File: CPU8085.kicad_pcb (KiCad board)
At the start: 2 copper layers, 100 x 100 mm, 52 parts, among them J1 USB_B, J2 SPEAKER, Q1 BC817, Q2 IRLML6402, SW1 RESET, U1 GLUE_LOGIC, U2 27C256, U3 IS61C256AH, U4 8250, U5 FT232RL, U6 82C54, U7 8085, U8 74LS573, Y1 4MHz

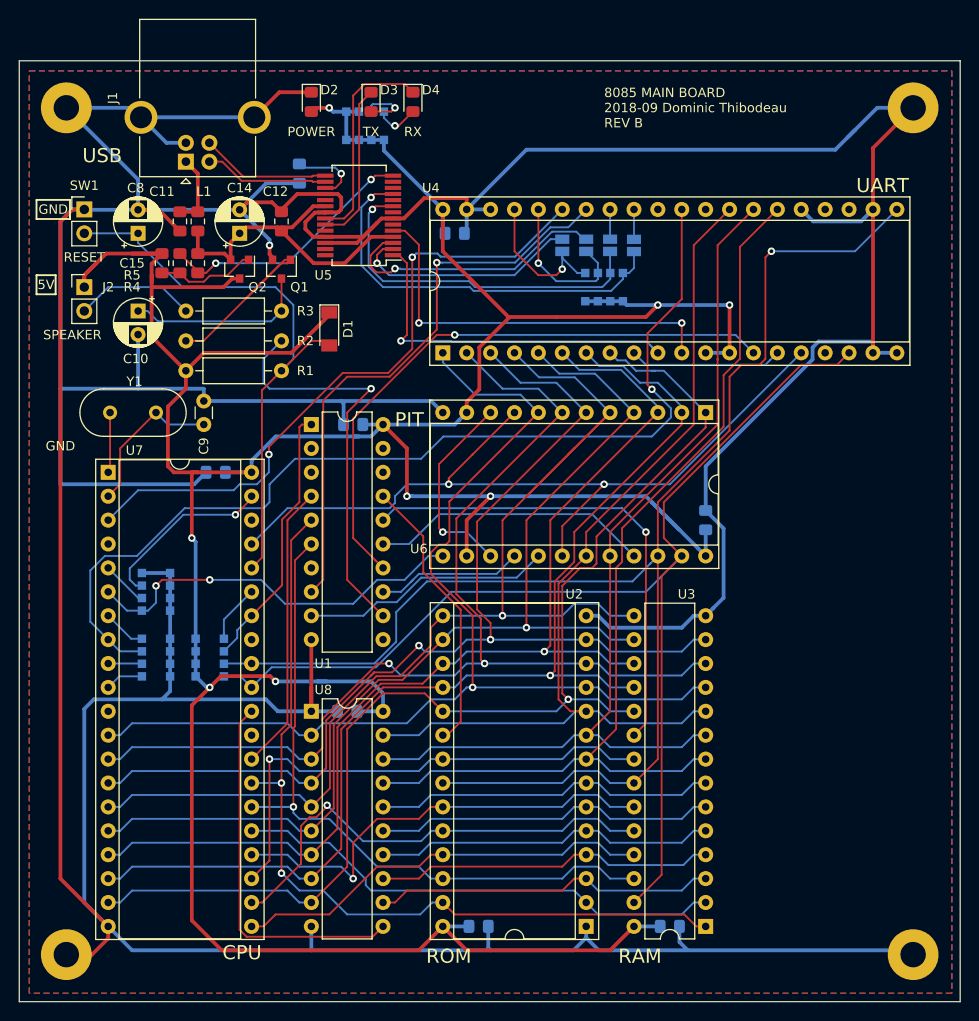
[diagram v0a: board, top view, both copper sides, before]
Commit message: RevC
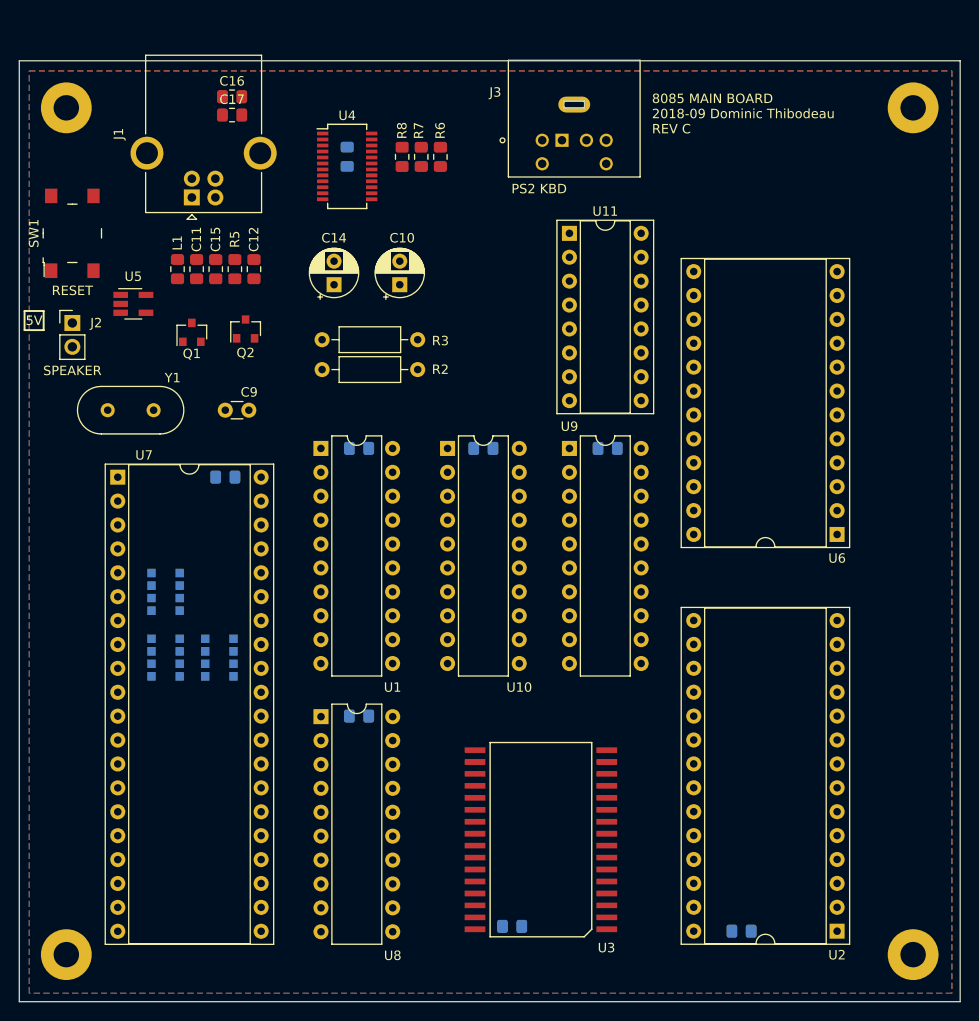
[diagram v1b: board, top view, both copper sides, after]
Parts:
- removed C8: 1uF, Capacitor_THT:CP_Radial_D5.0mm_P2.50mm
- removed D1: 1N4004, Diode_SMD:D_MiniMELF
- removed D2: POWER, LED_SMD:LED_0805_2012Metric_Pad1.15x1.40mm_HandSolder
- removed D3: TX, LED_SMD:LED_0805_2012Metric_Pad1.15x1.40mm_HandSolder
- removed D4: RX, LED_SMD:LED_0805_2012Metric_Pad1.15x1.40mm_HandSolder
- removed JP1: ~DTR, Jumper:SolderJumper-2_P1.3mm_Open_Pad1.0x1.5mm
- removed JP2: ~RTS, Jumper:SolderJumper-2_P1.3mm_Open_Pad1.0x1.5mm
- removed JP3: ~DSR, Jumper:SolderJumper-2_P1.3mm_Open_Pad1.0x1.5mm
- removed JP4: ~CTS, Jumper:SolderJumper-2_P1.3mm_Open_Pad1.0x1.5mm
- removed R1: 75K, Resistor_THT:R_Axial_DIN0207_L6.3mm_D2.5mm_P10.16mm_Horizontal
- removed R4: 10K, Resistor_SMD:R_0805_2012Metric_Pad1.15x1.40mm_HandSolder
- removed RN3: 10K, Resistor_SMD:R_Array_Convex_4x1206
- removed RN5: 330, Resistor_SMD:R_Array_Convex_4x1206
- added C16: 47pF, Capacitor_SMD:C_0805_2012Metric_Pad1.15x1.40mm_HandSolder, F.Cu at (57.6, 38.8)
- added C17: 47pF, Capacitor_SMD:C_0805_2012Metric_Pad1.15x1.40mm_HandSolder, F.Cu at (57.6, 40.8)
- added J3: PS2 KBD, 8085:CUI_MD-60S, F.Cu at (94.0, 41.1)
- added R6: 27R, Resistor_SMD:R_0805_2012Metric_Pad1.15x1.40mm_HandSolder, F.Cu at (79.8, 45.2)
- added R7: 27R, Resistor_SMD:R_0805_2012Metric_Pad1.15x1.40mm_HandSolder, F.Cu at (77.7, 45.2)
- added R8: 10K, Resistor_SMD:R_0805_2012Metric_Pad1.15x1.40mm_HandSolder, F.Cu at (75.7, 45.2)
- added U10: 74LS573, Package_DIP:DIP-20_W7.62mm, F.Cu at (80.5, 76.2)
- added U11: SN76489, Package_DIP:DIP-16_W7.62mm_Socket, F.Cu at (93.5, 53.3)
- added U9: DTBANK1, Package_DIP:DIP-20_W7.62mm, F.Cu at (93.5, 76.2)
- C12, C13: value 0.1uF -> 100nF
- C14: value 1uF -> 4.7uF
- SW1: footprint Connector_PinHeader_2.54mm:PinHeader_1x02_P2.54mm_Vertical -> 8085:Switch_Tactile_SMD_6x6mm_PTS645
- U1: value GLUE_LOGIC -> DTGLUE4
- U3: value IS61C256AH -> IS62C1024AL; footprint Package_DIP:DIP-28_W7.62mm -> 8085:SOIC-32W_14x21mm_P1.27mm
- U4: value 8250 -> FT240XS; footprint Package_DIP:DIP-40_W15.24mm_Socket -> Package_SO:SSOP-24_3.9x8.7mm_P0.635mm
- U5: value FT232RL -> MCP1319T-46LE; footprint Package_SO:SSOP-28_5.3x10.2mm_P0.65mm -> Package_TO_SOT_SMD:SOT-23-5_HandSoldering
- moved C4 67.8 mm to (111.8, 127.5), turned to 0 degrees
- moved C2 52.6 mm to (97.5, 76.2), turned to 180 degrees
- moved C6 37.6 mm to (71.1, 76.2), turned to 180 degrees
- moved C7 30.1 mm to (71.1, 104.6)
- moved C5 28.1 mm to (56.9, 79.2)
- moved C10 28.0 mm to (75.4, 58.8), turned to 90 degrees
- moved U2 26.7 mm to (121.9, 127.5)
- moved U5 25.8 mm to (47.1, 60.8), turned to 0 degrees
- moved R3 24.8 mm to (77.3, 64.6), turned to 180 degrees
- moved C1 23.1 mm to (84.3, 76.2), turned to 180 degrees
- moved U4 22.3 mm to (69.8, 46.2), turned to 0 degrees
- moved U3 19.8 mm to (90.4, 117.9)
- moved U6 19.1 mm to (121.9, 85.3), turned to 180 degrees
- moved C3 16.8 mm to (87.4, 127.0)
- moved R2 14.8 mm to (67.2, 67.8)
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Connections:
- net /UART/VIN renamed /UART (FT240XS)/VIN
- J1 pad 2: /UART/D- -> /UART (FT240XS)/D-
- J1 pad 3: /UART/D+ -> /UART (FT240XS)/D+
- R2 pad 2: /SPEAKER/SPKR_IN -> Net-(R2-Pad2)
- R5 pad 2: /UART/~PWREN -> /UART (FT240XS)/~PWREN
- RN1 pad 5: /PIT/TI_CLK -> /CPU/TRAP
- RN2 pad 7: /UART/INTR -> /CPU/RST6_5
- SW1 pad 2: Net-(C8-Pad1) -> Net-(SW1-Pad2)
- U1 pad 12: /SPEAKER/SPKR_IN -> (no net)
- U1 pad 13: /PIT/SPKR_EN -> (no net)
- U1 pad 14: /UART/~UART -> (no net)
- U1 pad 15: /PIT/~PIT -> /Sound (SN76489)/~SOUND
- U1 pad 16: /Memory/~RAMCE -> /UART (FT240XS)/~UART_RD
- U1 pad 17: /Memory/~ROMCE -> /UART (FT240XS)/UART_WR
- U1 pad 18: (no net) -> /PIT/~PIT
- U1 pad 19: (no net) -> /Memory/BANKREG
- U1 pad 2: (no net) -> /A15
- U1 pad 3: (no net) -> /A14
- U1 pad 4: /A15 -> /A13
- U1 pad 5: /A14 -> /CPU/~WR
- U1 pad 6: /A13 -> /CPU/~RD
- U1 pad 8: /UART/~UART_OUT1 -> (no net)
- U1 pad 9: /PIT/SPKR_OUT -> (no net)
- U3 pad 1: /A14 -> (no net)
- U3 pad 10: /CPU/A0 -> /CPU/A2
- U3 pad 11: /CPU/D0 -> /CPU/A1
- U3 pad 12: /CPU/D1 -> /CPU/A0
- U3 pad 13: /CPU/D2 -> /CPU/D0
- U3 pad 14: GND -> /CPU/D1
- U3 pad 15: /CPU/D3 -> /CPU/D2
- U3 pad 16: /CPU/D4 -> GND
- U3 pad 17: /CPU/D5 -> /CPU/D3
- U3 pad 18: /CPU/D6 -> /CPU/D4
- U3 pad 19: /CPU/D7 -> /CPU/D5
- U3 pad 2: /CPU/A12 -> /Memory/RAMA16
- U3 pad 20: /Memory/~RAMCE -> /CPU/D6
- U3 pad 21: /CPU/A10 -> /CPU/D7
- U3 pad 22: /CPU/~RD -> /Memory/~RAMCE
- U3 pad 23: /CPU/A11 -> /CPU/A10
- U3 pad 24: /CPU/A9 -> /CPU/~RD
- U3 pad 25: /CPU/A8 -> /CPU/A11
- U3 pad 26: /A13 -> /CPU/A9
- U3 pad 27: /CPU/~WR -> /CPU/A8
- U3 pad 28: VCC -> /Memory/RAMA13
- U3 pad 3: /CPU/A7 -> /Memory/RAMA14
- U3 pad 4: /CPU/A6 -> /CPU/A12
- U3 pad 5: /CPU/A5 -> /CPU/A7
- U3 pad 6: /CPU/A4 -> /CPU/A6
- U3 pad 7: /CPU/A3 -> /CPU/A5
- U3 pad 8: /CPU/A2 -> /CPU/A4
- U3 pad 9: /CPU/A1 -> /CPU/A3
- U4 pad 1: /CPU/D0 -> /CPU/D4
- U4 pad 11: Net-(U4-Pad11) -> /UART (FT240XS)/~UART_RD
- U4 pad 12: VCC -> /UART (FT240XS)/UART_WR
- U4 pad 13: VCC -> Net-(R6-Pad1)
- U4 pad 14: /UART/~UART -> Net-(R7-Pad1)
- U4 pad 15: Net-(U4-Pad15) -> Net-(C13-Pad1)
- U4 pad 16: /CPU/CLOCK -> Net-(C13-Pad1)
- U4 pad 18: /CPU/~WR -> VBUS
- U4 pad 2: /CPU/D1 -> /CPU/D2
- U4 pad 20: GND -> Net-(U4-Pad20)
- U4 pad 21: /CPU/~RD -> /CPU/SID
- U4 pad 22: GND -> Net-(U4-Pad22)
- U4 pad 23: Net-(U4-Pad23) -> /UART (FT240XS)/~PWREN
- U4 pad 24: Net-(U4-Pad24) -> /CPU/D0
- U4 pad 3: /CPU/D2 -> Net-(C13-Pad1)
- U4 pad 4: /CPU/D3 -> /CPU/D1
- U4 pad 5: /CPU/D4 -> /CPU/D7
- U4 pad 6: /CPU/D5 -> GND
- U4 pad 7: /CPU/D6 -> /CPU/D5
- U4 pad 8: /CPU/D7 -> /CPU/D6
- U4 pad 9: Net-(U4-Pad15) -> /CPU/D3
- U5 pad 1: Net-(U4-Pad10) -> Net-(U5-Pad1)
- U5 pad 2: Net-(JP3-Pad2) -> GND
- U5 pad 4: VBUS -> Net-(SW1-Pad2)
- U5 pad 5: Net-(U4-Pad11) -> VCC
- U6 pad 13: /PIT/TI_CLK -> /CPU/RST7_5
- U6 pad 16: /PIT/SPKR_EN -> VCC
- U6 pad 17: /PIT/SPKR_OUT -> Net-(U6-Pad17)
- U7 pad 36: Net-(C8-Pad1) -> Net-(U5-Pad1)
- U7 pad 6: /PIT/TI_CLK -> /CPU/TRAP
- U7 pad 8: /UART/INTR -> /CPU/RST6_5
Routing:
- net GND: track 645.6 -> 0.00 mm, vias 1 -> 0
- net VCC: track 392.8 -> 0.00 mm, vias 8 -> 0
- net /CPU/~RD: track 152.9 -> 0.00 mm, vias 1 -> 0
- net /CPU/D7: track 127.5 -> 0.00 mm, vias 1 -> 0
- net /CPU/~WR: track 126.6 -> 0.00 mm
- net /CPU/D3: track 124.2 -> 0.00 mm, vias 1 -> 0
- net /CPU/D6: track 120.7 -> 0.00 mm, vias 1 -> 0
- net /CPU/D2: track 118.2 -> 0.00 mm, vias 2 -> 0
- net /CPU/D1: track 118.1 -> 0.00 mm, vias 2 -> 0
- net /CPU/D0: track 117.3 -> 0.00 mm, vias 1 -> 0
- net /CPU/D5: track 116.3 -> 0.00 mm, vias 1 -> 0
- net /CPU/D4: track 112.0 -> 0.00 mm, vias 1 -> 0
- net /UART/INTR: track 106.4 -> 0.00 mm, vias 1 -> 0
- net /CPU/A2: track 103.7 -> 0.00 mm
- net /CPU/A1: track 99.8 -> 0.00 mm
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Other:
- board text added: "8085 MAIN BOARD 2018-09 Dominic Thibodeau REV C"
- board text removed: "8085 MAIN BOARD 2018-09 Dominic Thibodeau REV B"
- board text removed: "CPU"
- board text removed: "GND"
- board text removed: "PIT"
- board text removed: "POWER"
- board text removed: "RAM"
- board text removed: "ROM"
- board text removed: "RX"
- board text removed: "TX"
- board text removed: "UART"
- board text removed: "USB"
- board text removed: "~CTS"
- board text removed: "~DSR"
- board text removed: "~DTR"
- board text removed: "~RTS"
